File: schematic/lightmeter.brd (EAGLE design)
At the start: 27.9 x 52.6 mm, 80 parts, among them IC2 MCP73831/OT, J1 AVR_SPI_PRG_6NS, Q1 NCHANNELMOSFET, Q10 PCHANNELMOSFET, Q11 NCHANNELMOSFET, Q12 NCHANNELMOSFET, Q13 NCHANNELMOSFET, Q14 NCHANNELMOSFET, Q16 NCHANNELMOSFET, Q2 PCHANNELMOSFET, Q3 NCHANNELMOSFET, Q4 PCHANNELMOSFET, Q5 NCHANNELMOSFET, Q6 PCHANNELMOSFET, Q7 NCHANNELMOSFET, Q8 PCHANNELMOSFET, Q9 PCHANNELMOSFET

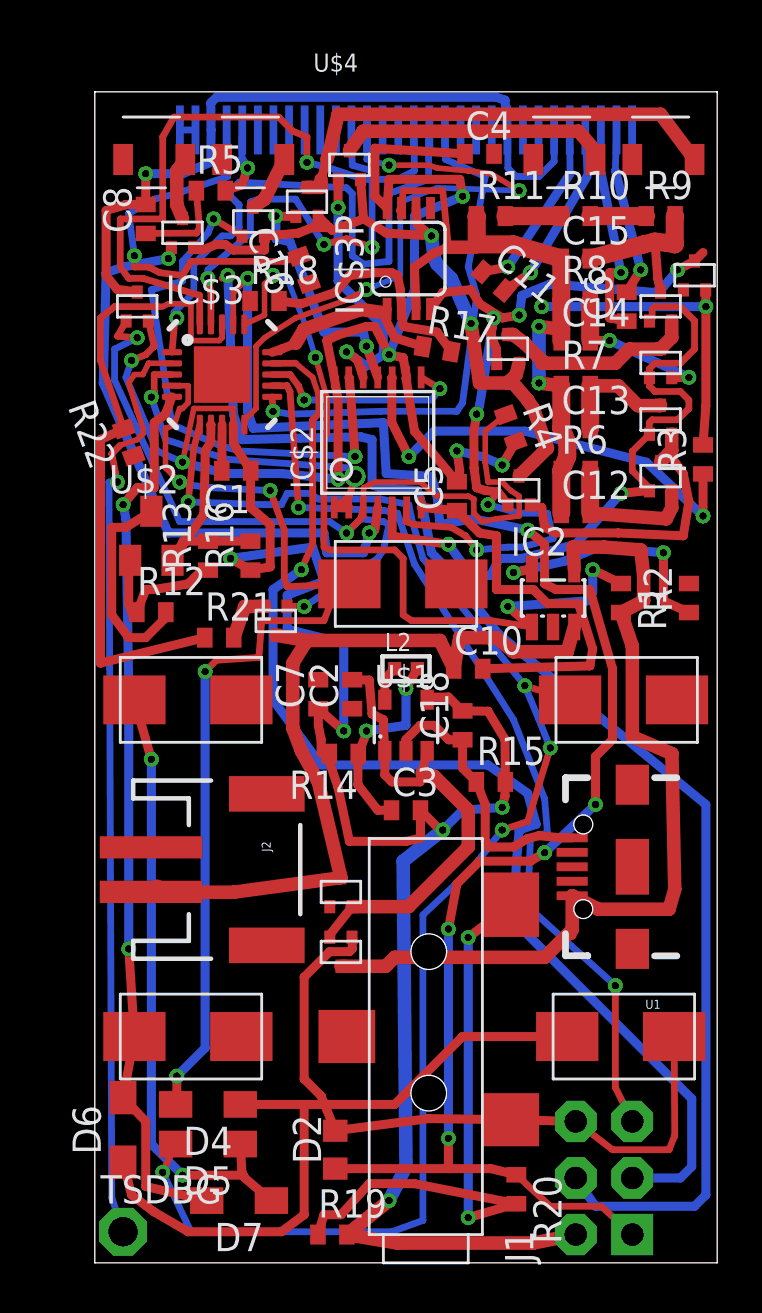
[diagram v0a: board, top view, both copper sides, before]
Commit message: Work on clearences.
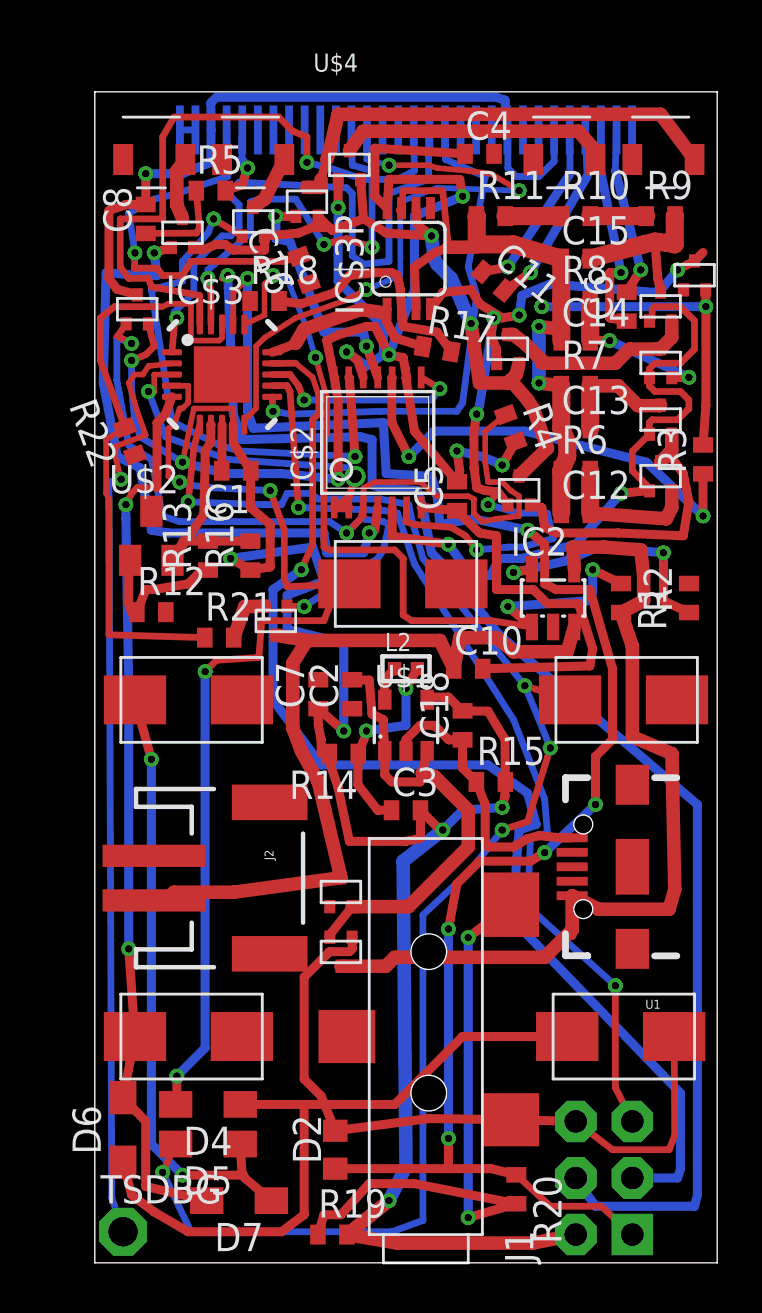
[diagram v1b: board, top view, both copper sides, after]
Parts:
- moved J2 0.40 mm to (5.08, 17.3)
- moved Q8 0.13 mm to (0.64, 43.1)
- moved R22 0.07 mm to (0.30, 36.9)
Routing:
- net GND: track 92.7 -> 83.3 mm
- net AVRMOSI/BATVOLTAGE: track 29.1 -> 27.2 mm
- net DIODESW$1: track 27.4 -> 29.0 mm
- net AVRSCK: track 54.3 -> 53.7 mm
